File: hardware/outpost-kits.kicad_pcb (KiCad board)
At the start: 2 copper layers, 105.8 x 102.7 mm, 28 parts, among them J1 PROBE, Q1 2N3904, SW1 ROLL, U1 NE555N, U2 CD4026, U3 SM420561N, U4 LM3915N

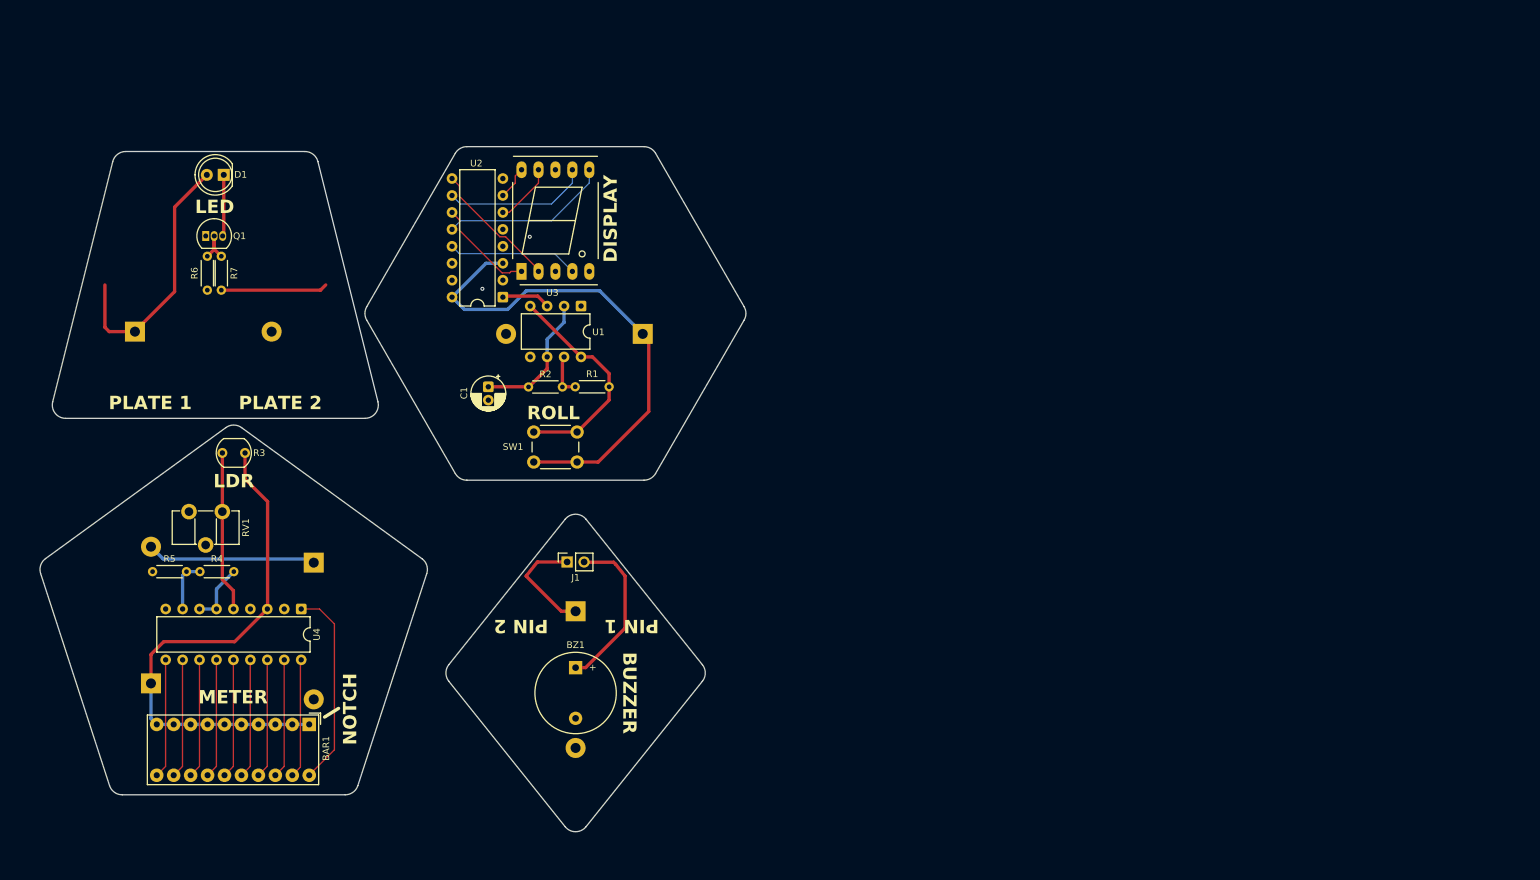
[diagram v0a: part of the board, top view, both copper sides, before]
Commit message: new panels + prod stuff
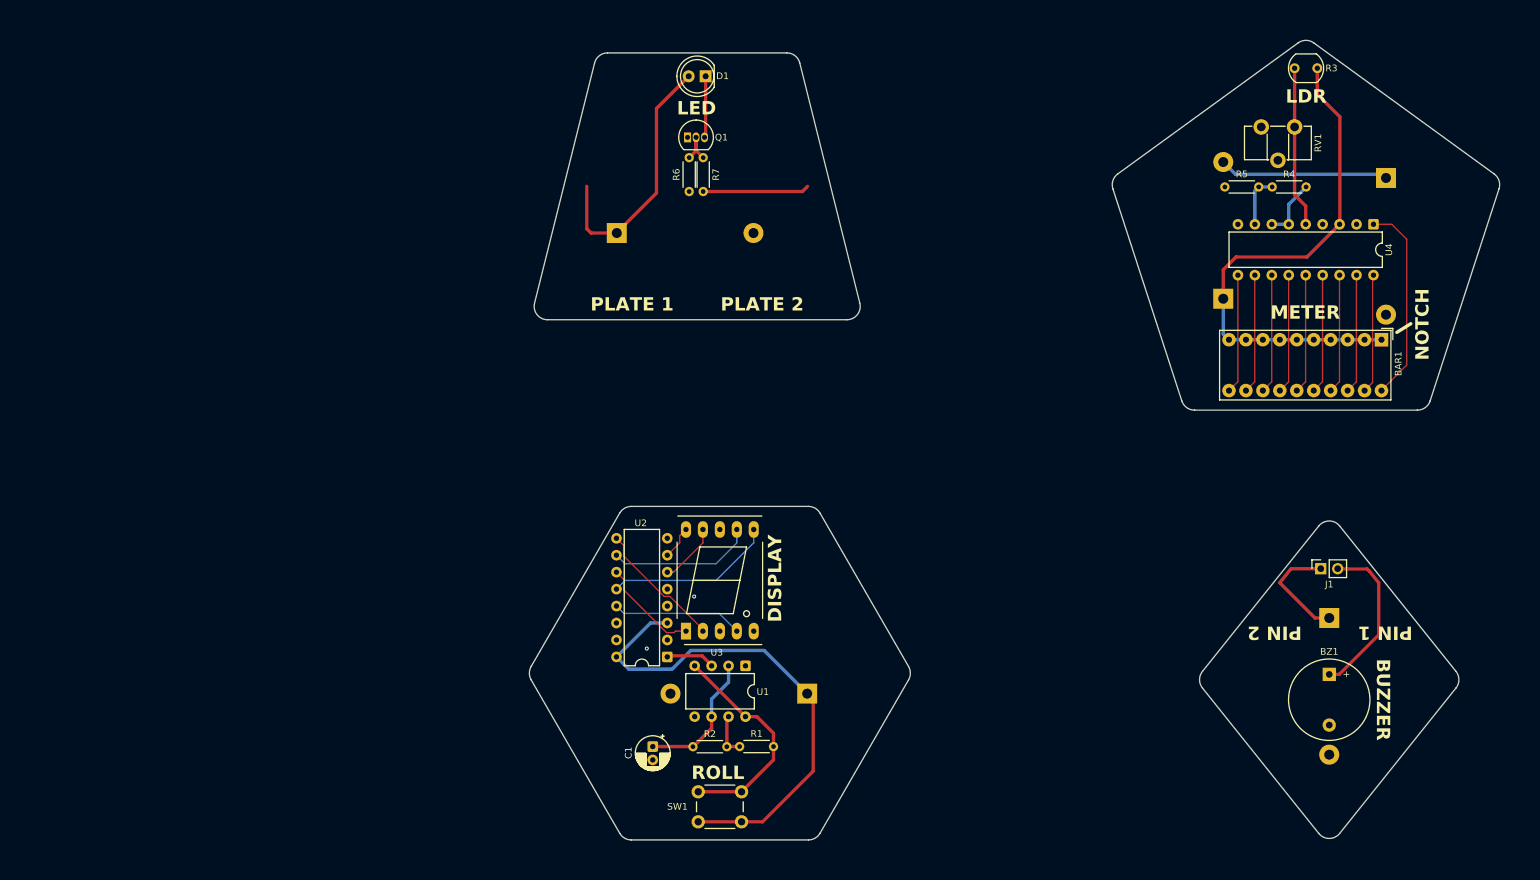
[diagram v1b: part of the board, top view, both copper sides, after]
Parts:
- moved BT1 170.8 mm to (234.7, 49.2)
- moved R4 170.8 mm to (217.6, 50.5)
- moved R5 170.8 mm to (210.5, 50.5)
- moved U4 170.8 mm to (232.8, 56.1)
- moved BAR1 170.8 mm to (234.0, 73.4)
- moved BT4 170.8 mm to (210.3, 67.3)
- moved G*** 170.8 mm to (215.7, 76.9)
- moved R3 170.8 mm to (224.4, 32.7)
- moved RV1 170.8 mm to (221.0, 41.5)
- moved BT3 113.0 mm to (226.1, 115.1)
- moved BZ1 113.0 mm to (226.2, 123.6)
- moved G*** 113.0 mm to (237.1, 119.7)
- moved J1 113.0 mm to (224.9, 107.8)
- moved G*** 73.7 mm to (131.9, 38.1)
- moved Q1 73.7 mm to (130.0, 43.1)
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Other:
- board size 105.8 x 102.7 mm -> 145.5 x 119.9 mm
